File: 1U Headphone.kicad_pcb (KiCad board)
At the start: 2 copper layers, 57.2 x 28.6 mm, 35 parts, among them J1 L IN, J2 R IN, J3 OUT, J4 Header_1x05, J5 Header_1x05, J6 Header_1x03, P1 A50k, U1 NJM2068

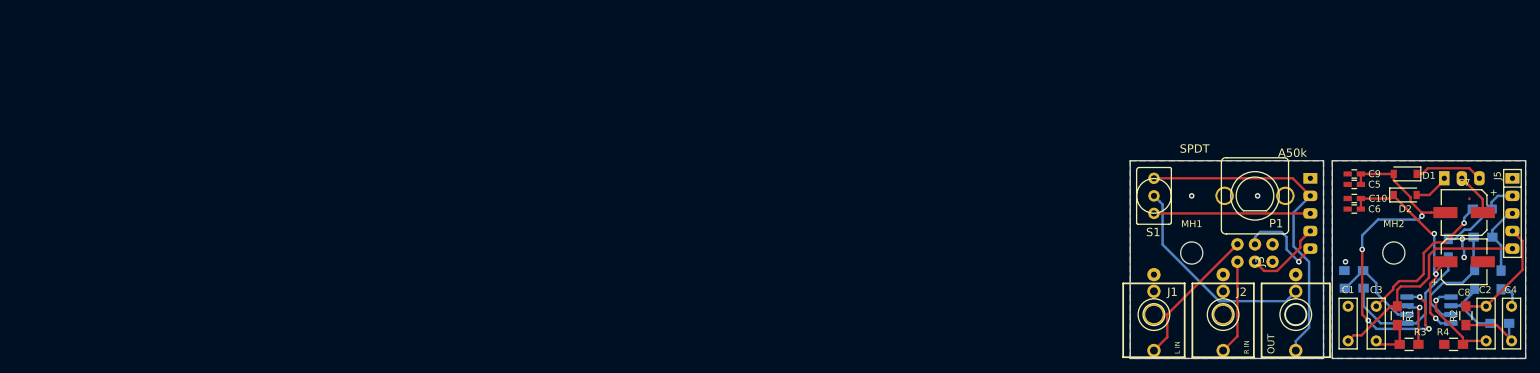
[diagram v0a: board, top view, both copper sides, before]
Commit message: Changed everything
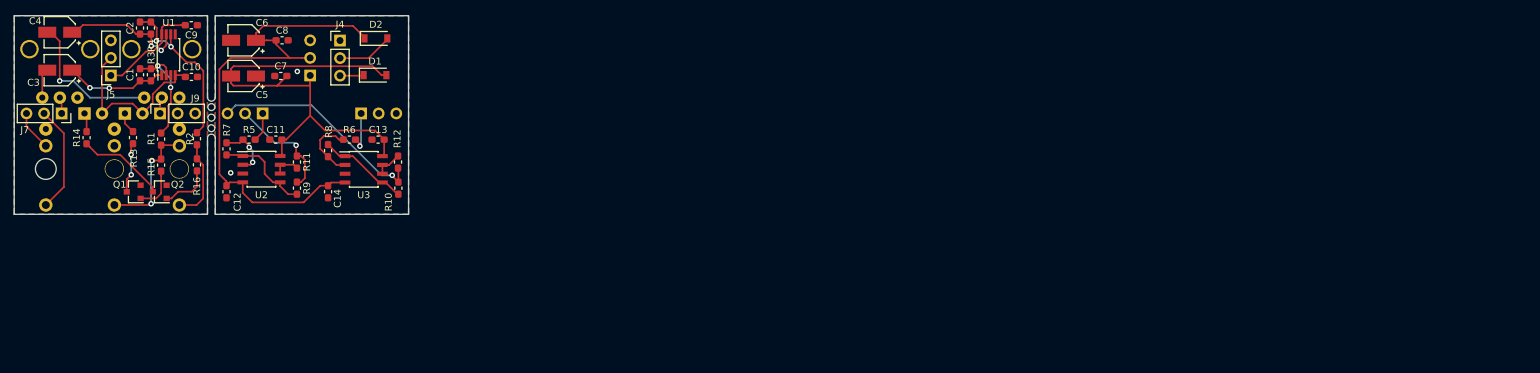
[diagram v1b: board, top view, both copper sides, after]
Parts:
- removed MH1, MH2: MountingHole, Mounting_Holes:MountingHole_3.2mm_M3
- removed P1: A50k, MojaBiblioteka:POT-9MM-ALPHA-DUAL
- removed R17, R18: R, Resistors_SMD:R_0805_HandSoldering
- removed S1: SPDT, 4ms-footprints:SPDT-SUB
- added C11: 100n, Capacitor_SMD:C_0603_1608Metric_Pad1.05x0.95mm_HandSolder, F.Cu at (55.6, 66.2)
- added C12: 100n, Capacitor_SMD:C_0603_1608Metric_Pad1.05x0.95mm_HandSolder, F.Cu at (48.5, 73.7)
- added C13: 100n, Capacitor_SMD:C_0603_1608Metric_Pad1.05x0.95mm_HandSolder, F.Cu at (70.4, 66.2)
- added C14: 100n, Capacitor_SMD:C_0603_1608Metric_Pad1.05x0.95mm_HandSolder, F.Cu at (63.1, 73.7)
- added D3: LED, LED_THT:LED_D3.0mm, B.Cu at (33.8, 62.4)
- added D4: LED, LED_THT:LED_D3.0mm, B.Cu at (27.9, 62.4)
- added J10: POT_L_M, Connector_PinHeader_2.54mm:PinHeader_1x03_P2.54mm_Vertical, B.Cu at (67.9, 62.4)
- added J7: POT_R_C, Connector_PinSocket_2.54mm:PinSocket_1x03_P2.54mm_Vertical, F.Cu at (24.6, 62.4)
- added J8: POT_R_M, Connector_PinHeader_2.54mm:PinHeader_1x03_P2.54mm_Vertical, B.Cu at (53.7, 62.4)
- added J9: POT_L_C, Connector_PinSocket_2.54mm:PinSocket_1x03_P2.54mm_Vertical, F.Cu at (38.9, 62.4)
- added Q1: MMBT3904, Package_TO_SOT_SMD:SOT-23, F.Cu at (35.1, 73.7)
- added Q2: MMBT3904, Package_TO_SOT_SMD:SOT-23, F.Cu at (38.8, 73.7)
- added R11: 75, Resistor_SMD:R_0603_1608Metric_Pad1.05x0.95mm_HandSolder, F.Cu at (58.6, 69.4)
- added R12: 75, Resistor_SMD:R_0603_1608Metric_Pad1.05x0.95mm_HandSolder, F.Cu at (73.3, 69.4)
- added R14: 1k, Resistor_SMD:R_0603_1608Metric_Pad1.05x0.95mm_HandSolder, F.Cu at (28.2, 65.9)
- added R16: 100k, Resistor_SMD:R_0603_1608Metric_Pad1.05x0.95mm_HandSolder, F.Cu at (44.2, 69.8)
- added R7: 10k, Resistor_SMD:R_0603_1608Metric_Pad1.05x0.95mm_HandSolder, F.Cu at (48.5, 67.5)
- added R8: 10k, Resistor_SMD:R_0603_1608Metric_Pad1.05x0.95mm_HandSolder, F.Cu at (63.1, 67.8)
- added RV1: 100k, KraakenStuff:POT-9MM-ALPHA, B.Cu at (24.4, 53.1)
- added RV2: 100k, KraakenStuff:POT-9MM-ALPHA, B.Cu at (39.1, 53.1)
- added U2: NE5532, Package_SO:SOIC-8_3.9x4.9mm_P1.27mm, F.Cu at (53.5, 70.4)
- added U3: NE5532, Package_SO:SOIC-8_3.9x4.9mm_P1.27mm, F.Cu at (68.3, 70.5)
- added ~: Perforacija, KraakenStuff:Perforacija, F.Cu at (46.3, 63.0)
- C1, C2: value 100n -> 10p; footprint Capacitors_THT:C_Rect_L7.2mm_W2.5mm_P5.00mm_FKS2_FKP2_MKS2_MKP2 -> Capacitor_SMD:C_0603_1608Metric_Pad1.05x0.95mm_HandSolder
- C10, C9: footprint Capacitors_SMD:C_0603_HandSoldering -> Capacitor_SMD:C_0603_1608Metric_Pad1.05x0.95mm_HandSolder
- C3, C4: value 100n -> 10uF; footprint Capacitors_THT:C_Rect_L7.2mm_W2.5mm_P5.00mm_FKS2_FKP2_MKS2_MKP2 -> Capacitor_SMD:CP_Elec_4x5.7
- C5, C6: value 100n -> 10uF; footprint Capacitors_SMD:C_0603_HandSoldering -> Capacitor_SMD:CP_Elec_4x5.7
- C7, C8: value 100u -> 100n; footprint Capacitors_SMD:CP_Elec_6.3x7.7 -> Capacitor_SMD:C_0603_1608Metric_Pad1.05x0.95mm_HandSolder
- D1, D2: footprint Diodes_SMD:D_SOD-123 -> Diode_SMD:D_SOD-123
- J1: value L IN -> R_IN; footprint 4ms-footprints:PJ301M-12 -> KraakenStuff:PJ301M-12; moved to B.Cu
- J2: value R IN -> L_IN; footprint 4ms-footprints:PJ301M-12 -> KraakenStuff:PJ301M-12; moved to B.Cu
- J3: footprint MojaBiblioteka:PJ366ST -> KraakenStuff:PJ366ST; moved to B.Cu
- J4: value Header_1x05 -> PWR; footprint MojaBiblioteka:Header 1x5 -> Connector_PinHeader_2.54mm:PinHeader_1x03_P2.54mm_Vertical; moved to F.Cu
- J5: value Header_1x05 -> PWR_C; footprint MojaBiblioteka:Header 1x5 -> Connector_PinSocket_2.54mm:PinSocket_1x03_P2.54mm_Vertical
- J6: value Header_1x03 -> PWR_M; footprint MojaBiblioteka:Header 1x3 -> Connector_PinHeader_2.54mm:PinHeader_1x03_P2.54mm_Vertical
- R1, R2: value R -> 100k; footprint Resistors_SMD:R_0805_HandSoldering -> Resistor_SMD:R_0603_1608Metric_Pad1.05x0.95mm_HandSolder
- R10, R9: value R -> 75; footprint Resistors_SMD:R_0805_HandSoldering -> Resistor_SMD:R_0603_1608Metric_Pad1.05x0.95mm_HandSolder; moved to F.Cu
- R13: value 68R/0.5W -> 1k; footprint Resistors_SMD:R_0805_HandSoldering -> Resistor_SMD:R_0603_1608Metric_Pad1.05x0.95mm_HandSolder; moved to F.Cu
- R15: value 68R/0.5W -> 100k; footprint Resistors_SMD:R_0805_HandSoldering -> Resistor_SMD:R_0603_1608Metric_Pad1.05x0.95mm_HandSolder; moved to F.Cu
- R3, R4: value 100k -> 39k; footprint Resistors_SMD:R_0805_HandSoldering -> Resistor_SMD:R_0603_1608Metric_Pad1.05x0.95mm_HandSolder
- R5, R6: value R -> 10k; footprint Resistors_SMD:R_0805_HandSoldering -> Resistor_SMD:R_0603_1608Metric_Pad1.05x0.95mm_HandSolder; moved to F.Cu
- U1: value NJM2068 -> TL072; footprint 4ms-footprints:DMP8 -> Package_SO:TSSOP-8_4.4x3mm_P0.65mm; moved to F.Cu
- moved C4 214.5 mm to (24.4, 50.6), turned to 180 degrees
- moved J5 203.5 mm to (31.8, 56.9), turned to 180 degrees
- moved C2 199.7 mm to (36.0, 50.0)
- moved C3 194.2 mm to (24.4, 56.1), turned to 180 degrees
- moved R4 193.7 mm to (37.5, 50.0), turned to 90 degrees
- moved R15 191.3 mm to (39.0, 69.8), turned to 270 degrees
- moved R13 190.8 mm to (35.0, 65.9), turned to 90 degrees
- moved R3 186.0 mm to (37.5, 56.8), turned to 90 degrees
- moved U1 185.9 mm to (40.1, 53.9), turned to 90 degrees
- moved R2 185.2 mm to (44.2, 66.0)
- moved J3 181.9 mm to (22.4, 70.4)
- moved R1 180.5 mm to (39.0, 66.1)
- moved C1 177.8 mm to (36.0, 56.8), turned to 90 degrees
- moved C8 173.8 mm to (56.5, 51.8)
- moved C7 172.2 mm to (56.3, 57.0), turned to 0 degrees
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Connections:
- C1 pad 2: L_IN -> Net-(C1-Pad2)
- C2 pad 2: R_IN -> Net-(C2-Pad2)
- C3 pad 1: GND -> Net-(C1-Pad1)
- C4 pad 1: GND -> Net-(C2-Pad1)
- J4 pad 2: L_OUT -> Net-(D2-Pad2)
- J4 pad 3: R_OUT -> Net-(D1-Pad1)
- J5 pad 1: GND -> -12V
- J5 pad 2: L_OUT -> +12V
- J5 pad 3: R_OUT -> GND
- J6 pad 1: Net-(D2-Pad2) -> -12V
- J6 pad 2: GND -> +12V
- J6 pad 3: Net-(D1-Pad1) -> GND
- R1 pad 1: L_IN -> Net-(C1-Pad2)
- R1 pad 2: GND -> Net-(J1-PadT)
- R10 pad 1: GND -> OUT_L_M
- R13 pad 1: L_OUT -> Net-(Q1-Pad3)
- R13 pad 2: Net-(R13-Pad2) -> Net-(D3-Pad1)
- R15 pad 1: R_OUT -> Net-(J1-PadT)
- R15 pad 2: Net-(R15-Pad2) -> Net-(Q1-Pad1)
- R2 pad 1: R_IN -> Net-(C2-Pad2)
- R2 pad 2: GND -> Net-(J2-PadT)
- R3 pad 2: GND -> Net-(C1-Pad2)
- R4 pad 2: GND -> Net-(C2-Pad2)
- R5 pad 1: Net-(R13-Pad2) -> Net-(R5-Pad1)
- R5 pad 2: Net-(R5-Pad2) -> POT_R_M
- R6 pad 1: GND -> Net-(R6-Pad1)
- R6 pad 2: Net-(R5-Pad2) -> POT_L_M
- R9 pad 1: Net-(R15-Pad2) -> OUT_R_M
- R9 pad 2: Net-(R10-Pad2) -> Net-(R7-Pad1)
- U1 pad 1: Net-(R13-Pad2) -> Net-(C1-Pad1)
- U1 pad 2: Net-(R5-Pad2) -> Net-(C1-Pad2)
- U1 pad 3: Net-(C1-Pad1) -> GND
- U1 pad 4: -12V -> +12V
- U1 pad 5: Net-(C2-Pad1) -> GND
- U1 pad 6: Net-(R10-Pad2) -> Net-(C2-Pad2)
- U1 pad 7: Net-(R15-Pad2) -> Net-(C2-Pad1)
- U1 pad 8: +12V -> -12V
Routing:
- net +12V: track 32.9 -> 101.4 mm, vias 3 -> 0
- net L_OUT: track 61.2 -> 0.00 mm
- net L_IN: track 45.7 -> 0.00 mm, vias 1 -> 0
- net R_OUT: track 32.9 -> 0.00 mm
- net OUT_L_M: track 0.00 -> 31.9 mm, vias 0 -> 1
- net Net-(J3-Pad2): track 30.8 -> 0.00 mm
- net R_IN: track 28.1 -> 0.00 mm
- net GND: track 26.0 -> 0.00 mm, vias 5 -> 2
- net -12V: track 56.8 -> 82.8 mm, vias 5 -> 0
- net Net-(C2-Pad2): track 0.00 -> 24.4 mm, vias 0 -> 2
- net Net-(R13-Pad2): track 22.6 -> 0.00 mm
- net Net-(J1-Pad3): track 20.3 -> 0.00 mm
- net Net-(C3-Pad2): track 22.2 -> 4.26 mm, vias 1 -> 0
- net Net-(J1-PadT): track 0.00 -> 17.8 mm, vias 0 -> 2
- net Net-(C4-Pad2): track 3.73 -> 21.3 mm, vias 0 -> 1
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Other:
- board size 57.2 x 28.6 mm -> 57 x 28.7 mm
- net class Default: clearance 0.25 -> 0.2; trace_width 0.35 -> 0.25
- rule pad_to_mask_clearance: 0.2 -> 0
- rule trace_clearance: 0.25 -> 0.2
- board text added: "KraakenStuff Headphone v.0.1"
- board text removed: "Kraaken Headphone v0.1"
